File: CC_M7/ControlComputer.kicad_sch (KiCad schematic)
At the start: 39 parts, among them U1 STM32H743VGTx, Y1 32MHz

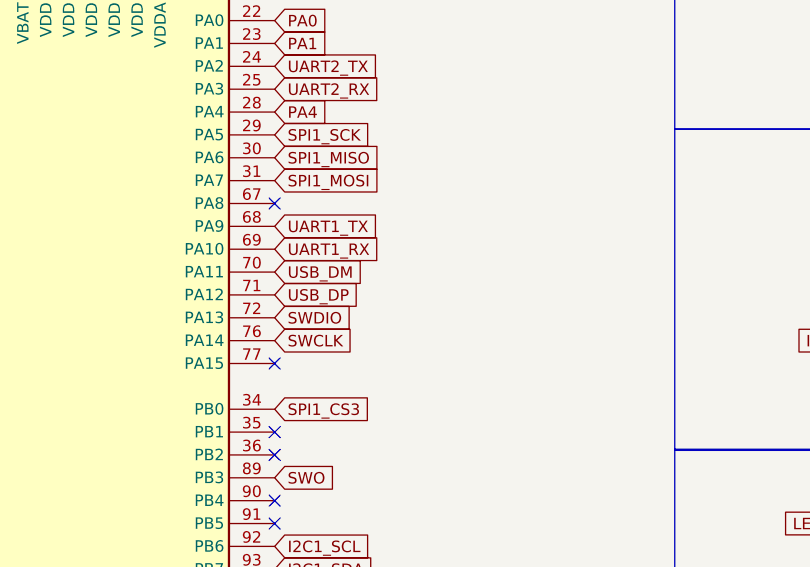
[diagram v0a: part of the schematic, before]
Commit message: last check
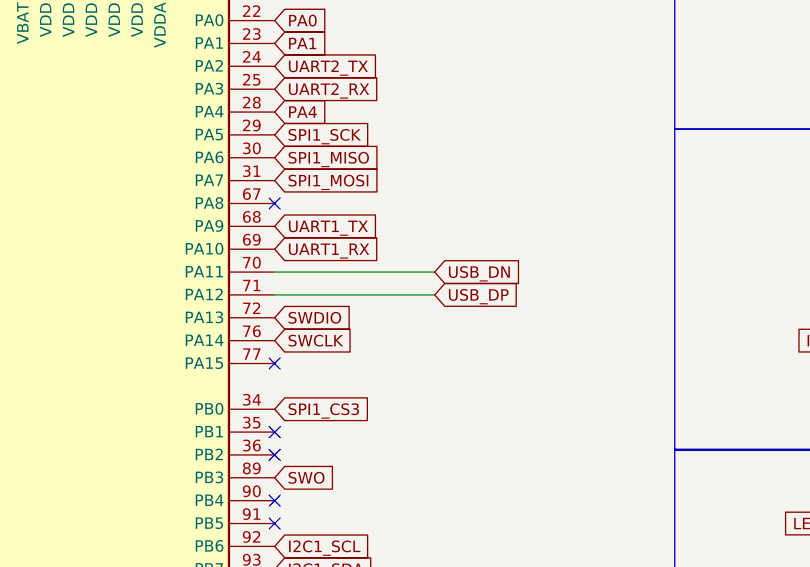
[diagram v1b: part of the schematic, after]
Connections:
- net USB_DM renamed USB_DN
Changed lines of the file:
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@@
+	(wire
+		(pts
+			(xy 106.68 139.7) (xy 88.9 139.7)
+		)
+		(stroke
+			(width 0)
+			(type default)
+		)
+	)
 	(wire
 		(pts
@@
 		(pts
 			(xy 165.1 35.56) (xy 165.1 38.1)
+		)
+		(stroke
+			(width 0)
+			(type default)
+		)
+	)
+	(wire
+		(pts
+			(xy 106.68 142.24) (xy 88.9 142.24)
 		)
 		(stroke
@@
 		)
 	)
-	(global_label "USB_DM"
-		(shape input)
-		(at 88.9 139.7 0)
-		(fields_autoplaced yes)
-		(effects
-			(font
-				(size 1.27 1.27)
-			)
-			(justify left)
-		)
-		(property "Intersheetrefs" "${INTERSHEET_REFS}"
-			(at 99.3842 139.7 0)
-			(effects
-				(font
-					(size 1.27 1.27)
-				)
-				(justify left)
-				(hide yes)
-			)
-		)
-	)
 	(global_label "TIM3_CH1"
 		(shape input)
@@
 		)
 	)
+	(global_label "USB_DN"
+		(shape input)
+		(at 106.68 139.7 0)
+		(fields_autoplaced yes)
+		(effects
+			(font
+				(size 1.27 1.27)
+			)
+			(justify left)
+		)
+		(property "Intersheetrefs" "${INTERSHEET_REFS}"
+			(at 117.0433 139.7 0)
+			(effects
+				(font
+					(size 1.27 1.27)
+				)
+				(justify left)
+				(hide yes)
+			)
+		)
+	)
 	(global_label "PE2"
 		(shape input)
@@
 	(global_label "USB_DP"
 		(shape input)
-		(at 88.9 142.24 0)
-		(fields_autoplaced yes)
-		(effects
-			(font
-				(size 1.27 1.27)
-			)
-			(justify left)
-		)
-		(property "Intersheetrefs" "${INTERSHEET_REFS}"
-			(at 99.2028 142.24 0)
-			(effects
-				(font
+		(at 106.68 142.24 0)
+		(fields_autoplaced yes)
+		(effects
+			(font
+				(size 1.27 1.27)
+			)
+			(justify left)
+		)
+		(property "Intersheetrefs" "${INTERSHEET_REFS}"
+			(at 116.9828 142.24 0)
+			(effects
+				(font
